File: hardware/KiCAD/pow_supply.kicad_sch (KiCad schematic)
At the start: 18 parts, among them U8 TPS563208, U9 TPS563208

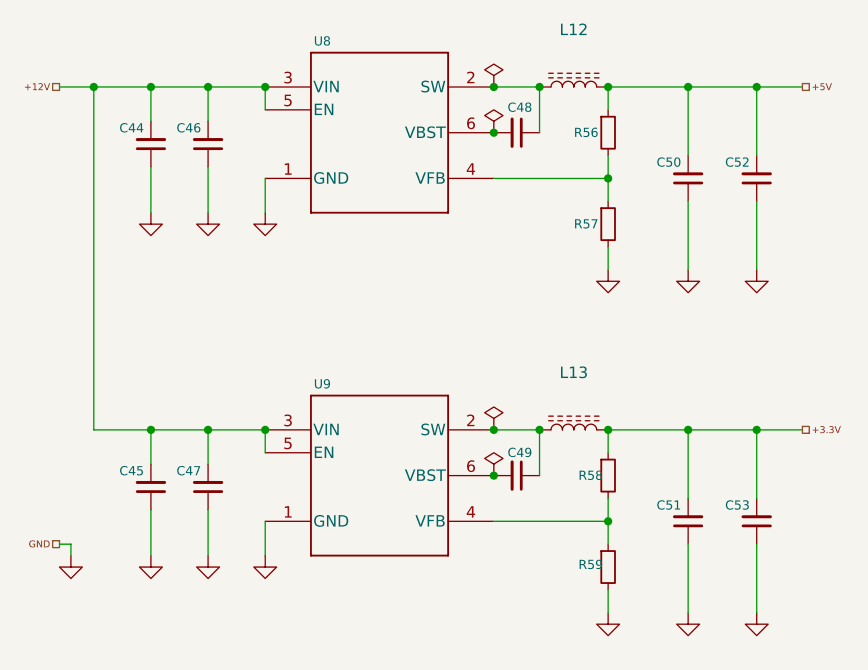
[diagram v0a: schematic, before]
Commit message: update
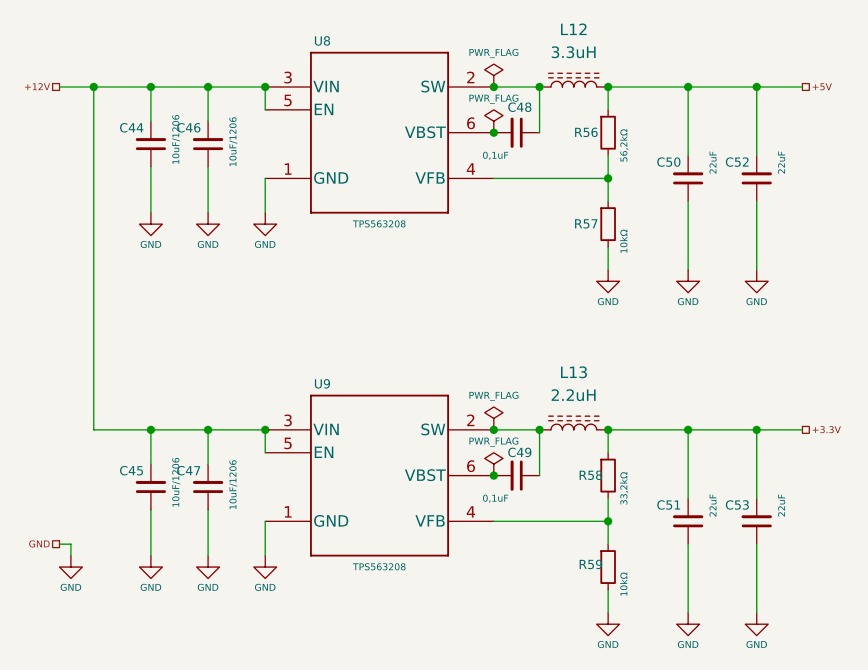
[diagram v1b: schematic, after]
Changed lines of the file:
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@@
 					(size 0.762 0.762)
 				)
-				(hide yes)
 			)
 		)
@@
 				)
 				(justify left)
-				(hide yes)
 			)
 		)
@@
 					(size 0.762 0.762)
 				)
-				(hide yes)
 			)
 		)
@@
 				)
 				(justify left)
-				(hide yes)
 			)
 		)
@@
 				)
 				(justify left)
-				(hide yes)
 			)
 		)
@@
 					(size 0.762 0.762)
 				)
-				(hide yes)
 			)
 		)
@@
 					(size 0.762 0.762)
 				)
-				(hide yes)
 			)
 		)
@@
 				)
 				(justify left)
-				(hide yes)
 			)
 		)
@@
 				)
 				(justify left)
-				(hide yes)
 			)
 		)
@@
 					(size 0.762 0.762)
 				)
-				(hide yes)
 			)
 		)
@@
 				)
 				(justify left)
-				(hide yes)
 			)
 		)
@@
 				)
 				(justify left)
-				(hide yes)
 			)
 		)
@@
 				)
 				(justify left)
-				(hide yes)
 			)
 		)
@@
 					(size 1.27 1.27)
 				)
-				(hide yes)
 			)
 		)
@@
 				)
 				(justify left)
-				(hide yes)
 			)
 		)
@@
 					(size 0.762 0.762)
 				)
-				(hide yes)
 			)
 		)
@@
 				)
 				(justify left)
-				(hide yes)
 			)
 		)
@@
 					(size 0.762 0.762)
 				)
-				(hide yes)
 			)
 		)
@@
 					(size 0.762 0.762)
 				)
-				(hide yes)
 			)
 		)
@@
 					(size 0.762 0.762)
 				)
-				(hide yes)
 			)
 		)
@@
 					(size 0.762 0.762)
 				)
-				(hide yes)
 			)
 		)
@@
 					(size 0.762 0.762)
 				)
-				(hide yes)
 			)
 		)
@@
 				)
 				(justify left)
-				(hide yes)
 			)
 		)
@@
 					(size 0.762 0.762)
 				)
-				(hide yes)
 			)
 		)
@@
 					(size 0.762 0.762)
 				)
-				(hide yes)
 			)
 		)
@@
 					(size 0.762 0.762)
 				)
-				(hide yes)
 			)
 		)
@@
 					(size 0.762 0.762)
 				)
-				(hide yes)
 			)
 		)
@@
 					(size 0.762 0.762)
 				)
-				(hide yes)
 			)
 		)
@@
 					(size 0.762 0.762)
 				)
-				(hide yes)
 			)
 		)
@@
 				)
 				(justify left)
-				(hide yes)
 			)
 		)
@@
 					(size 1.27 1.27)
 				)
-				(hide yes)
 			)
 		)
@@
 					(size 0.762 0.762)
 				)
-				(hide yes)
 			)
 		)
@@
 				)
 				(justify left)
-				(hide yes)
 			)
 		)
@@
 					(size 0.762 0.762)
 				)
-				(hide yes)
 			)
 		)
@@
 				)
 				(justify left)
-				(hide yes)
 			)
 		)

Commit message: update
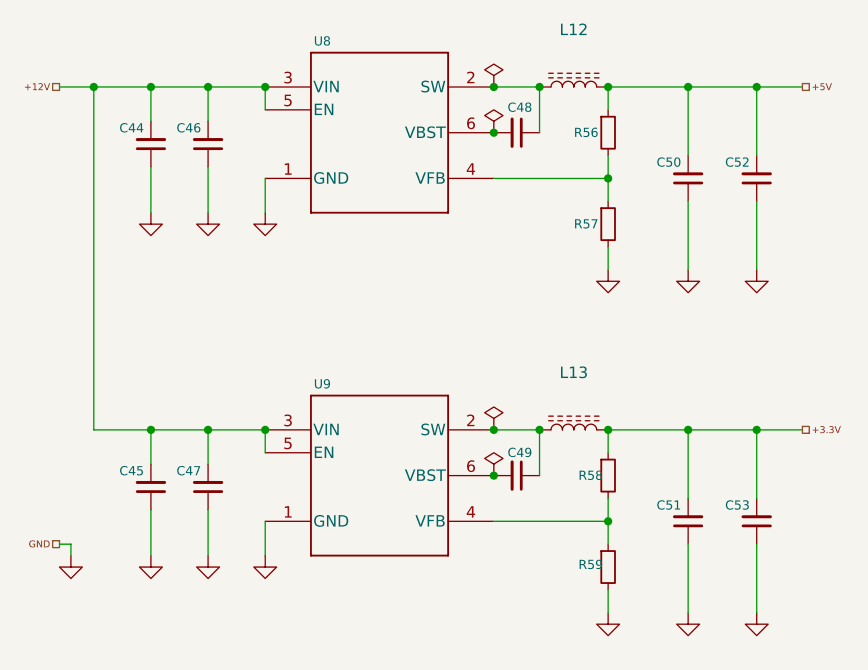
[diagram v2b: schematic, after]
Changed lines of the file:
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@@
 					(size 0.762 0.762)
 				)
+				(hide yes)
 			)
 		)
@@
 				)
 				(justify left)
+				(hide yes)
 			)
 		)
@@
 					(size 0.762 0.762)
 				)
+				(hide yes)
 			)
 		)
@@
 				)
 				(justify left)
+				(hide yes)
 			)
 		)
@@
 				)
 				(justify left)
+				(hide yes)
 			)
 		)
@@
 					(size 0.762 0.762)
 				)
+				(hide yes)
 			)
 		)
@@
 					(size 0.762 0.762)
 				)
+				(hide yes)
 			)
 		)
@@
 				)
 				(justify left)
+				(hide yes)
 			)
 		)
@@
 				)
 				(justify left)
+				(hide yes)
 			)
 		)
@@
 					(size 0.762 0.762)
 				)
+				(hide yes)
 			)
 		)
@@
 				)
 				(justify left)
+				(hide yes)
 			)
 		)
@@
 				)
 				(justify left)
+				(hide yes)
 			)
 		)
@@
 				)
 				(justify left)
+				(hide yes)
 			)
 		)
@@
 					(size 1.27 1.27)
 				)
+				(hide yes)
 			)
 		)
@@
 				)
 				(justify left)
+				(hide yes)
 			)
 		)
@@
 					(size 0.762 0.762)
 				)
+				(hide yes)
 			)
 		)
@@
 				)
 				(justify left)
+				(hide yes)
 			)
 		)
@@
 					(size 0.762 0.762)
 				)
+				(hide yes)
 			)
 		)
@@
 					(size 0.762 0.762)
 				)
+				(hide yes)
 			)
 		)
@@
 					(size 0.762 0.762)
 				)
+				(hide yes)
 			)
 		)
@@
 					(size 0.762 0.762)
 				)
+				(hide yes)
 			)
 		)
@@
 					(size 0.762 0.762)
 				)
+				(hide yes)
 			)
 		)
@@
 				)
 				(justify left)
+				(hide yes)
 			)
 		)
@@
 					(size 0.762 0.762)
 				)
+				(hide yes)
 			)
 		)
@@
 					(size 0.762 0.762)
 				)
+				(hide yes)
 			)
 		)
@@
 					(size 0.762 0.762)
 				)
+				(hide yes)
 			)
 		)
@@
 					(size 0.762 0.762)
 				)
+				(hide yes)
 			)
 		)
@@
 					(size 0.762 0.762)
 				)
+				(hide yes)
 			)
 		)
@@
 					(size 0.762 0.762)
 				)
+				(hide yes)
 			)
 		)
@@
 				)
 				(justify left)
+				(hide yes)
 			)
 		)
@@
 					(size 1.27 1.27)
 				)
+				(hide yes)
 			)
 		)
@@
 					(size 0.762 0.762)
 				)
+				(hide yes)
 			)
 		)
@@
 				)
 				(justify left)
+				(hide yes)
 			)
 		)
@@
 					(size 0.762 0.762)
 				)
+				(hide yes)
 			)
 		)
@@
 				)
 				(justify left)
+				(hide yes)
 			)
 		)
